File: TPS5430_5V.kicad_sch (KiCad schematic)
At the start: 12 parts, among them U1 TPS5430DDA, U2 Output, U3 Input

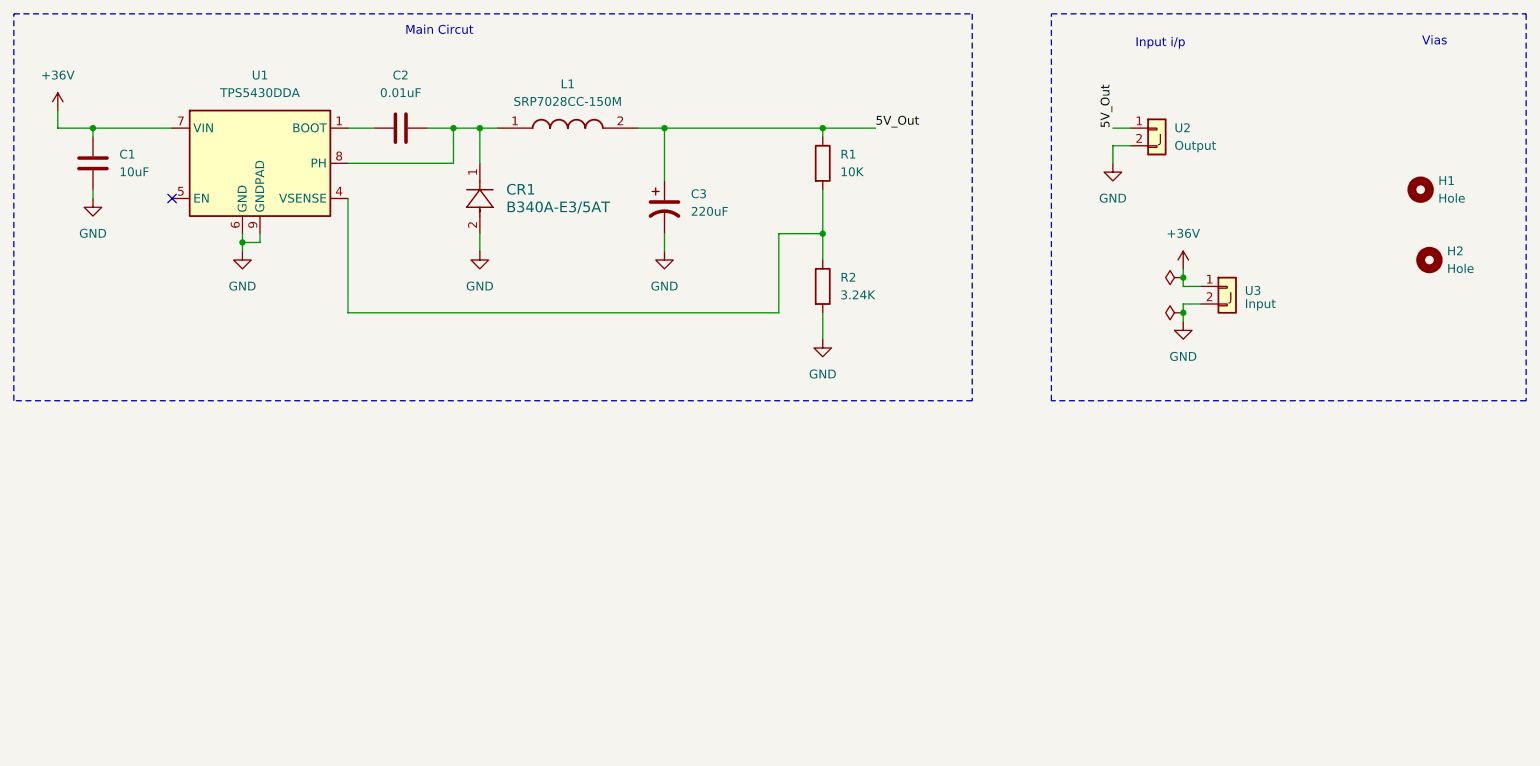
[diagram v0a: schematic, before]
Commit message: New Updation
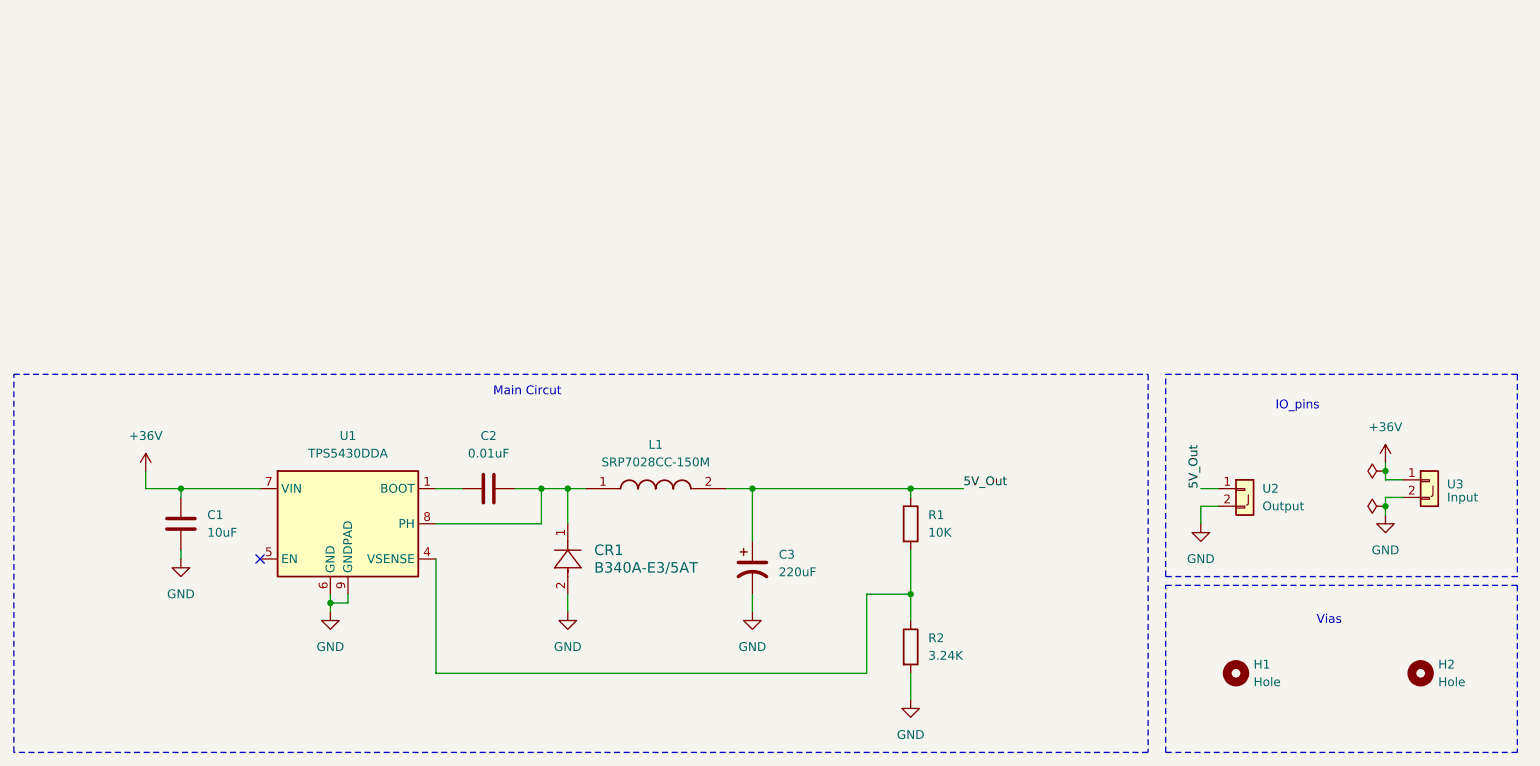
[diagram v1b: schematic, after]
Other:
- note added: "IO_pins"
- note removed: "Input i/p"
- moved on the sheet: C1, C2, C3, CR1, H1, H2, L1, R1, R2, U1, U2, U3
